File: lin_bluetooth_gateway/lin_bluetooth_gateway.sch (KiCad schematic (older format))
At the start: 9 parts, among them P1 CONN_01X01, P2 CONN_01X01, P3 CONN_01X01, P4 CONN_01X03, U1 MCP2050, U2 BL652

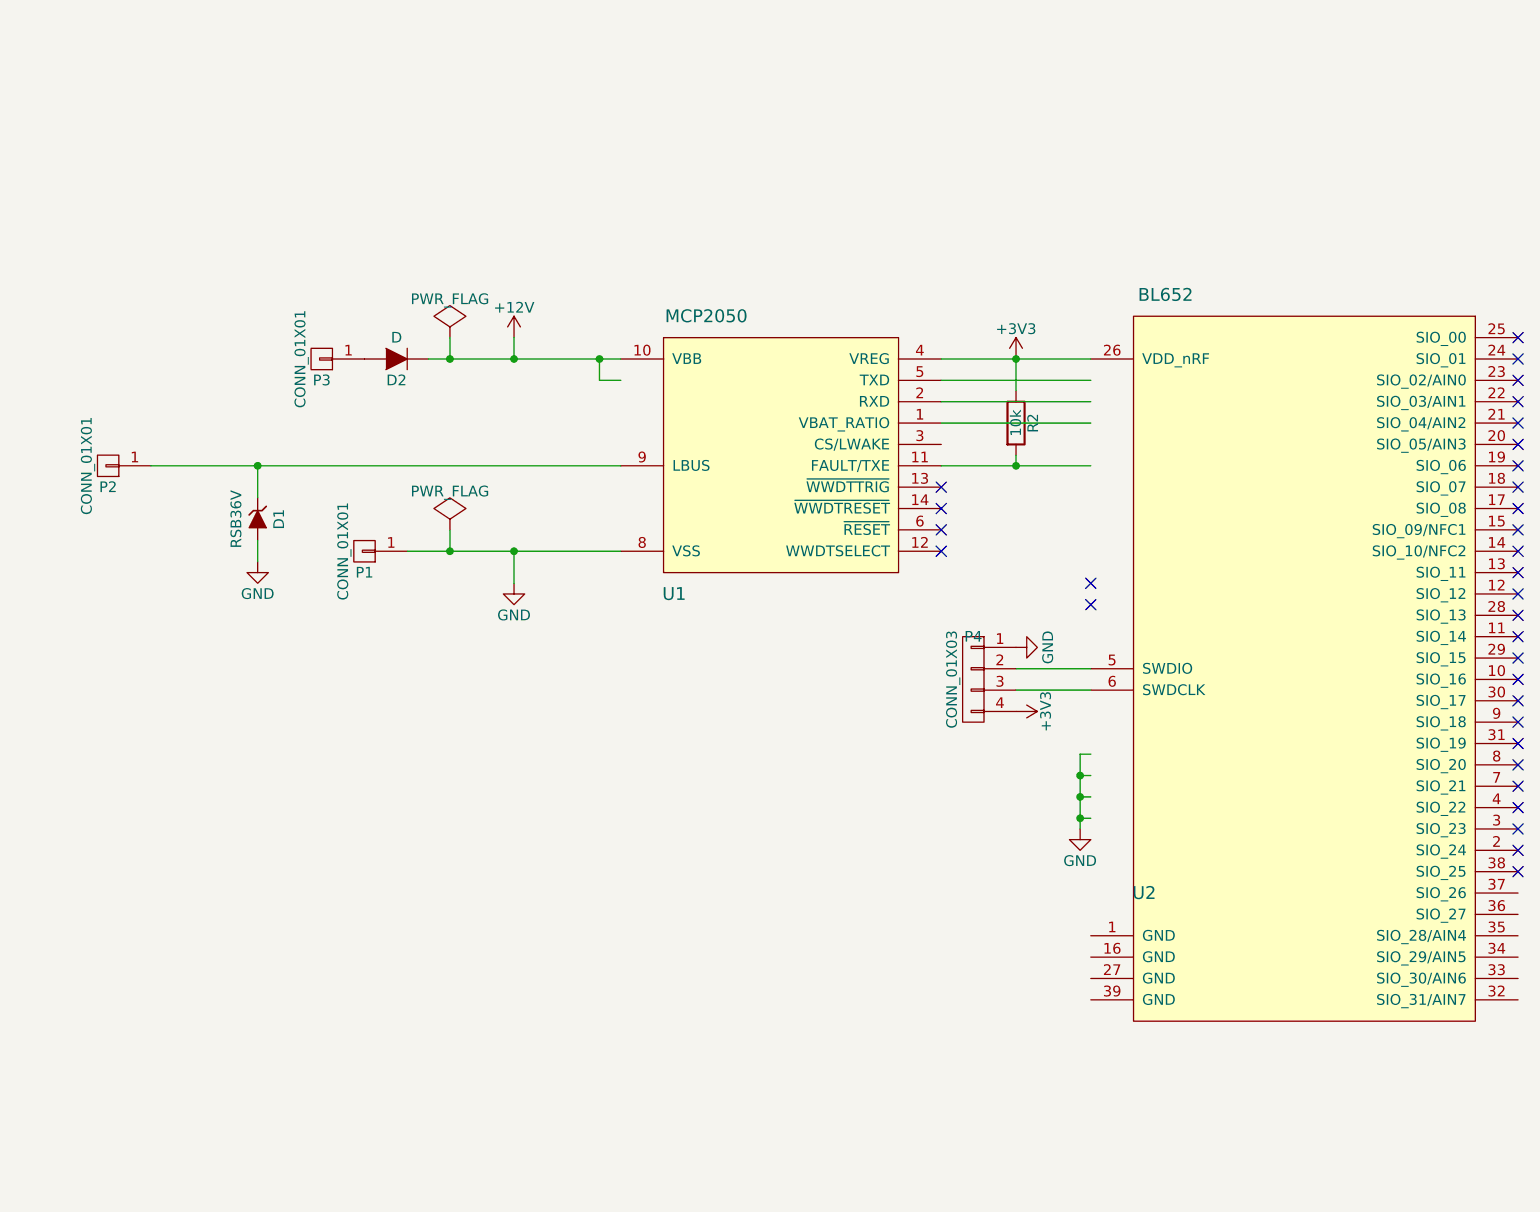
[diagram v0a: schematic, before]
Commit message: lin_bluetooth_gateway rev2
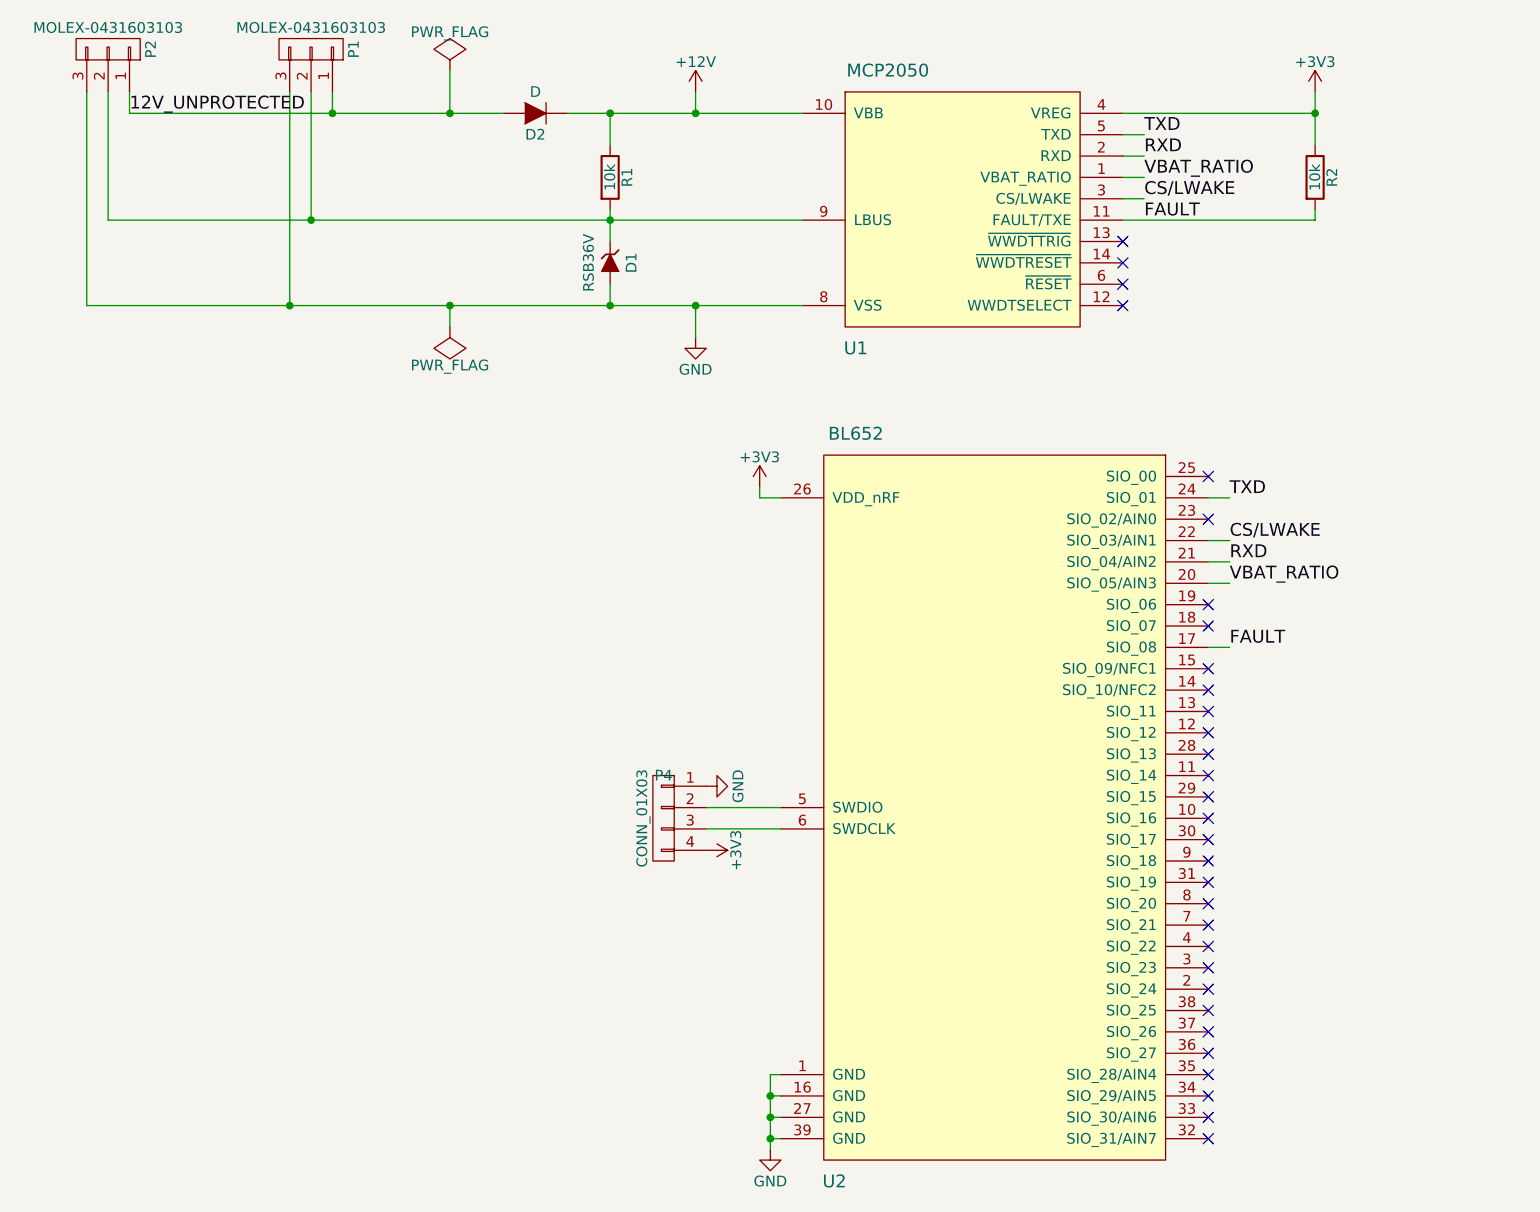
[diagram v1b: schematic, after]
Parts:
- removed P1, P2, P3: CONN_01X01, Wire_Pads:SolderWirePad_single_1-2mmDrill, symbol CONN_01X01
- added P1, P2: MOLEX-0431603103, Connectors_Molex:Molex_Sabre_43160-XX03_03x7.49mm_Angled_BoardLock, symbol CONN_01X03
- added R1: 10k, Resistors_SMD:R_0603_HandSoldering, symbol R
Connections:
- net labels added: 12V_UNPROTECTED, CS/LWAKE, FAULT, RXD, TXD, VBAT_RATIO
- wire segments 25 -> 39
- no-connect marks 32 -> 31
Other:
- moved on the sheet: D1, D2, P4, R2, U1, U2
